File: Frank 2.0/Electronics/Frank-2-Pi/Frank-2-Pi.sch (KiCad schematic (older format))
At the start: 11 parts, among them J2 Left motor, J3 Right motor, Q1 DMN6075S, Q2 DMN6075S, U1 adafruit-2448

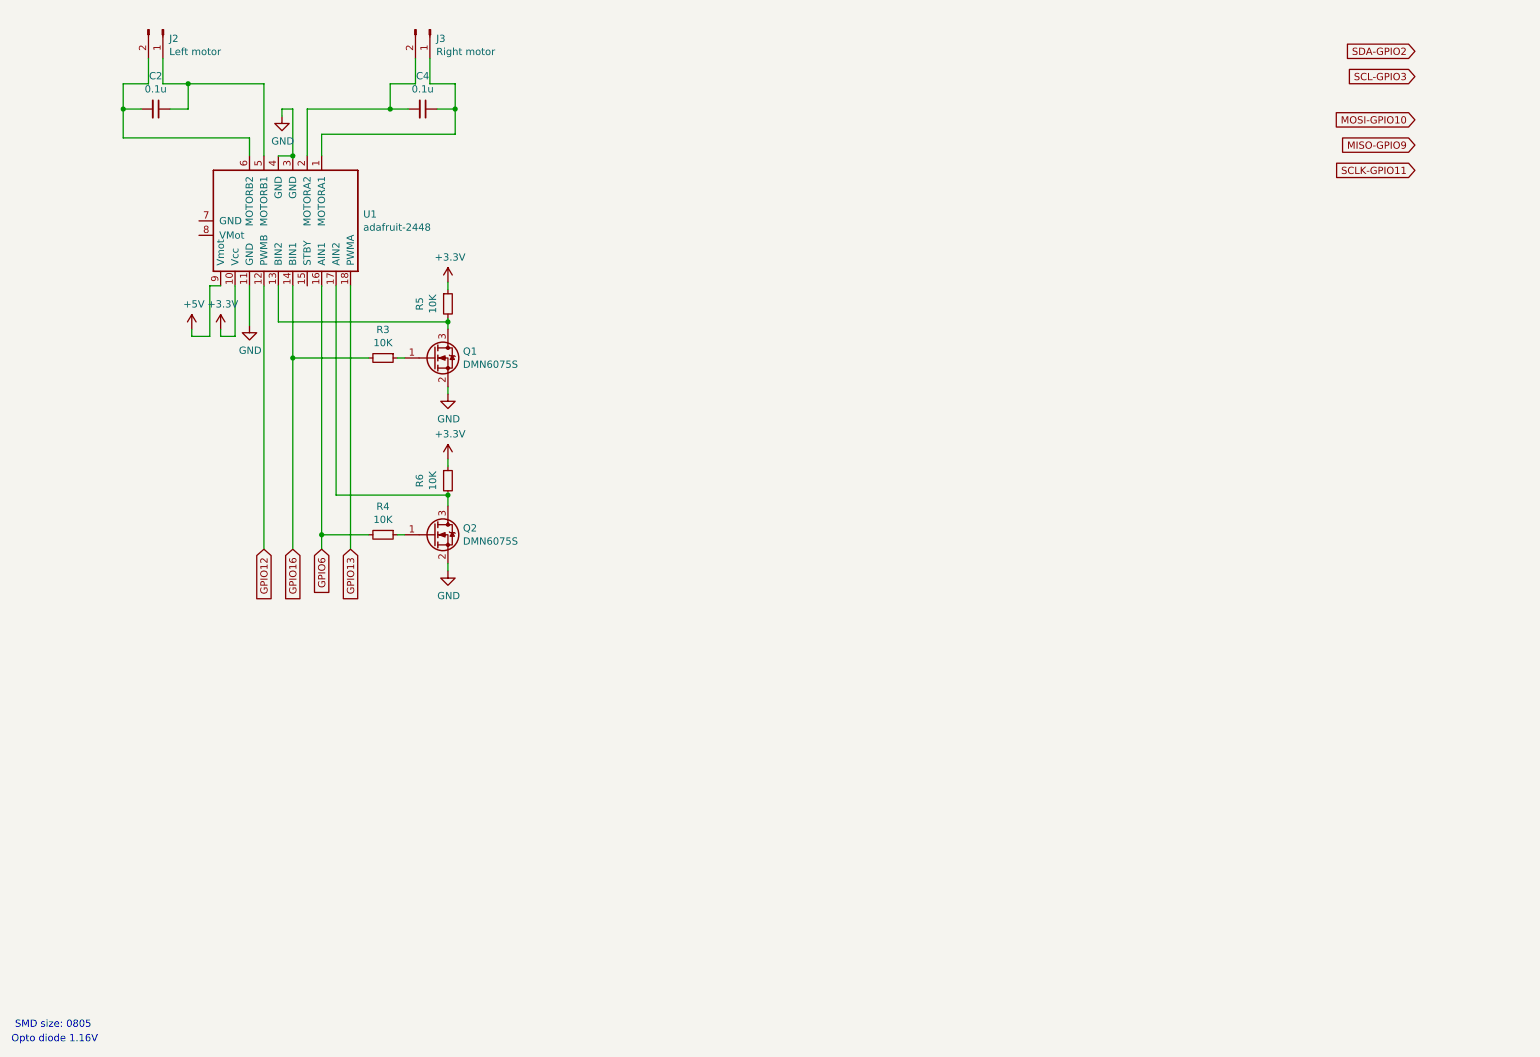
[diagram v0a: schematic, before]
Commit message: Frank 2 electronics WIP.
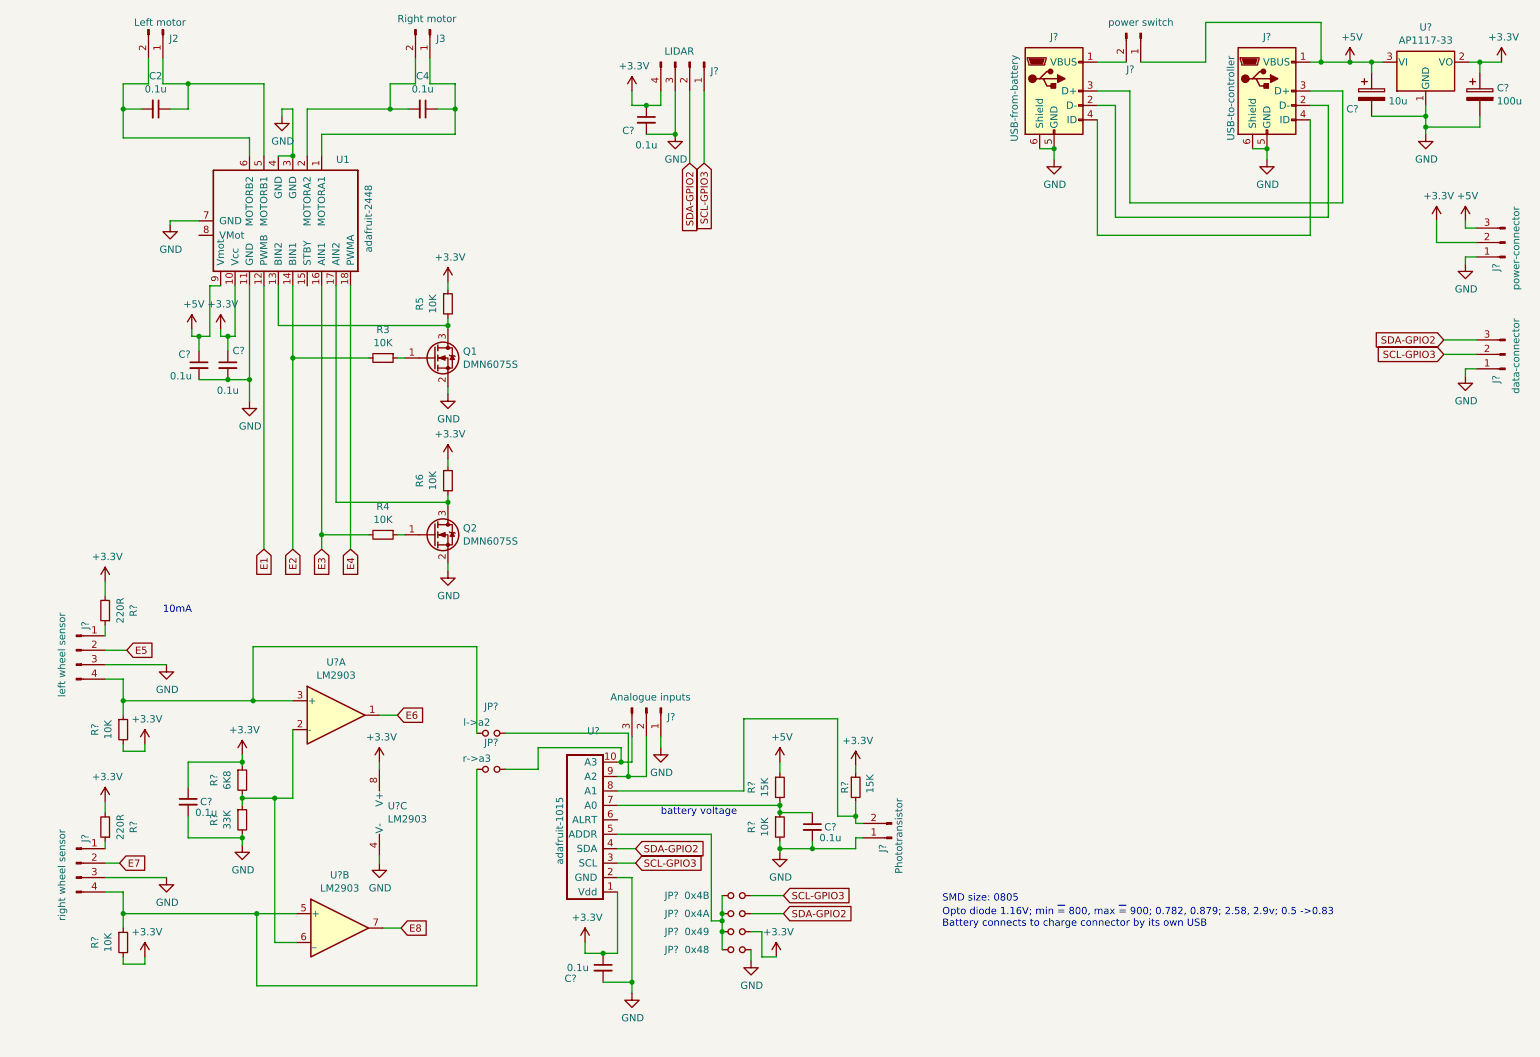
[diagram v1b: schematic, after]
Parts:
- added C? (x6): 0.1u, Capacitor_SMD:C_0805_2012Metric, symbol Device:C_Small
- added C?: 10u, Capacitor_Tantalum_SMD:CP_EIA-3216-18_Kemet-A_Pad1.58x1.35mm_HandSolder, symbol Device:CP
- added C?: 100u, Capacitor_Tantalum_SMD:CP_EIA-3216-18_Kemet-A_Pad1.58x1.35mm_HandSolder, symbol Device:CP
- added J?: LIDAR, Connector_PinHeader_2.54mm:PinHeader_1x04_P2.54mm_Vertical, symbol Connector:Conn_01x04_Male
- added J?: left wheel sensor, Connector_PinHeader_2.54mm:PinHeader_1x04_P2.54mm_Vertical, symbol Connector:Conn_01x04_Male
- added J?: Phototransistor, Connector_PinHeader_2.54mm:PinHeader_1x02_P2.54mm_Vertical, symbol Connector:Conn_01x02_Male
- added J?: Analogue inputs, Connector_PinHeader_2.54mm:PinHeader_1x03_P2.54mm_Vertical, symbol Connector:Conn_01x03_Male
- added J?: right wheel sensor, Connector_PinHeader_2.54mm:PinHeader_1x04_P2.54mm_Vertical, symbol Connector:Conn_01x04_Male
- added J?: USB-to-controller, Connector_USB:USB_Micro-B_Wuerth_629105150521, symbol Connector:USB_OTG
- added J?: USB-from-battery, Connector_USB:USB_Micro-B_Wuerth_629105150521, symbol Connector:USB_OTG
- added J?: power switch, Connector_PinHeader_2.54mm:PinHeader_1x02_P2.54mm_Vertical, symbol Connector:Conn_01x02_Male
- added J?: power-connector, Connector_PinHeader_2.54mm:PinHeader_1x03_P2.54mm_Vertical, symbol Connector:Conn_01x03_Male
- added J?: data-connector, Connector_PinHeader_2.54mm:PinHeader_1x03_P2.54mm_Vertical, symbol Connector:Conn_01x03_Male
- added JP?: 0x48, Jumper:SolderJumper-2_P1.3mm_Open_RoundedPad1.0x1.5mm, symbol Device:Jumper_NO_Small
- added JP?: 0x49, Jumper:SolderJumper-2_P1.3mm_Open_RoundedPad1.0x1.5mm, symbol Device:Jumper_NO_Small
- added JP?: 0x4A, Jumper:SolderJumper-2_P1.3mm_Open_RoundedPad1.0x1.5mm, symbol Device:Jumper_NO_Small
- added JP?: 0x4B, Jumper:SolderJumper-2_P1.3mm_Open_RoundedPad1.0x1.5mm, symbol Device:Jumper_NO_Small
- added JP?: l->a2, Jumper:SolderJumper-2_P1.3mm_Open_RoundedPad1.0x1.5mm, symbol Device:Jumper_NO_Small
- added JP?: r->a3, Jumper:SolderJumper-2_P1.3mm_Open_RoundedPad1.0x1.5mm, symbol Device:Jumper_NO_Small
- added R? (x2): 220R, Resistor_SMD:R_0805_2012Metric, symbol Device:R_Small
- added R? (x3): 10K, Resistor_SMD:R_0805_2012Metric, symbol Device:R_Small
- added R?: 6K8, Resistor_SMD:R_0805_2012Metric, symbol Device:R_Small
- added R?: 33K, Resistor_SMD:R_0805_2012Metric, symbol Device:R_Small
- added R? (x2): 15K, Resistor_SMD:R_0805_2012Metric, symbol Device:R_Small
- added U? (x3): LM2903, Package_SO:Diodes_SO-8EP, symbol Comparator:LM2903
- added U?: adafruit-1015, reprapltd-kicad:adafruit-1015, symbol reprapltd-kicad:adafruit-1015
- added U?: AP1117-33, Package_TO_SOT_SMD:SOT-223-3_TabPin2, symbol Regulator_Linear:AP1117-33
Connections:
- net +3V3: now also C?.1, C?.1, C?.1, C?.1, C?.1, J?.2 (Pin_2), J?.4 (Pin_4), JP?.2, R?.1, R?.1, R?.2, R?.2, R?.2, R?.2, U?.1 (Vdd), U?.2 (VO), U?.8 (V+)
- net +5V: now also C?.1, C?.1, J?.1 (Pin_1), J?.1 (VBUS), J?.3 (Pin_3), R?.1, U?.3 (VI)
- net GND: now also U1.7 (GND), C?.2, C?.2, C?.2, C?.2, C?.2, C?.2, C?.2, C?.2, J?.1 (Pin_1), J?.1 (Pin_1), J?.1 (Pin_1), J?.1 (Pin_1), J?.3 (Pin_3), J?.3 (Pin_3), J?.3 (Pin_3), J?.5 (GND), J?.5 (GND), J?.6 (Shield), J?.6 (Shield), JP?.2, R?.2, R?.2, U?.1 (GND), U?.2 (GND), U?.4 (V-)
- net SCL-GPIO3: now also J?.1 (Pin_1), J?.2 (Pin_2), JP?.2, U?.3 (SCL)
- net SDA-GPIO2: now also J?.2 (Pin_2), J?.3 (Pin_3), JP?.2, U?.4 (SDA)
- net GPIO12 renamed E1
- net GPIO13 renamed E4
- net GPIO16 renamed E2
- net GPIO6 renamed E3
- new net: J?.1 (Pin_1), R?.1 (x2)
- new net: JP?.1, JP?.1, JP?.1, JP?.1, U?.5 (ADDR)
- new net: J?.4 (Pin_4), JP?.1, R?.1, U?.3 (+)
- new net: J?.4 (Pin_4), JP?.1, R?.1, U?.5 (+)
- new net: R?.1, R?.2, U?.2 (-), U?.6 (_)
- new net: J?.3 (Pin_3), JP?.2, U?.10 (A3)
- new net: C?.1, R?.1, R?.2, U?.7 (A0)
- new net: J?.2 (Pin_2), R?.2, U?.8 (A1)
- new net: J?.2 (Pin_2), JP?.2, U?.9 (A2)
- new net: J?.2 (D-), J?.2 (D-)
- new net: J?.3 (D+), J?.3 (D+)
- new net: J?.4 (ID), J?.4 (ID)
- new net: J?.1 (VBUS), J?.2 (Pin_2)
- new net E5: J?.2 (Pin_2)
- new net E6: U?.1
- new net E7: J?.2 (Pin_2)
- new net E8: U?.7
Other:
- note added: "10mA"
- note added: "Opto diode 1.16V; min ~= 800, max ~= 900; 0.782, 0.879; 2.58, 2.9v; 0.5 ->0.83\nBattery connects to charge connector by its own USB"
- note added: "battery voltage"
- note removed: "Opto diode 1.16V"

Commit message: Frank 2.0 electronics WIP.
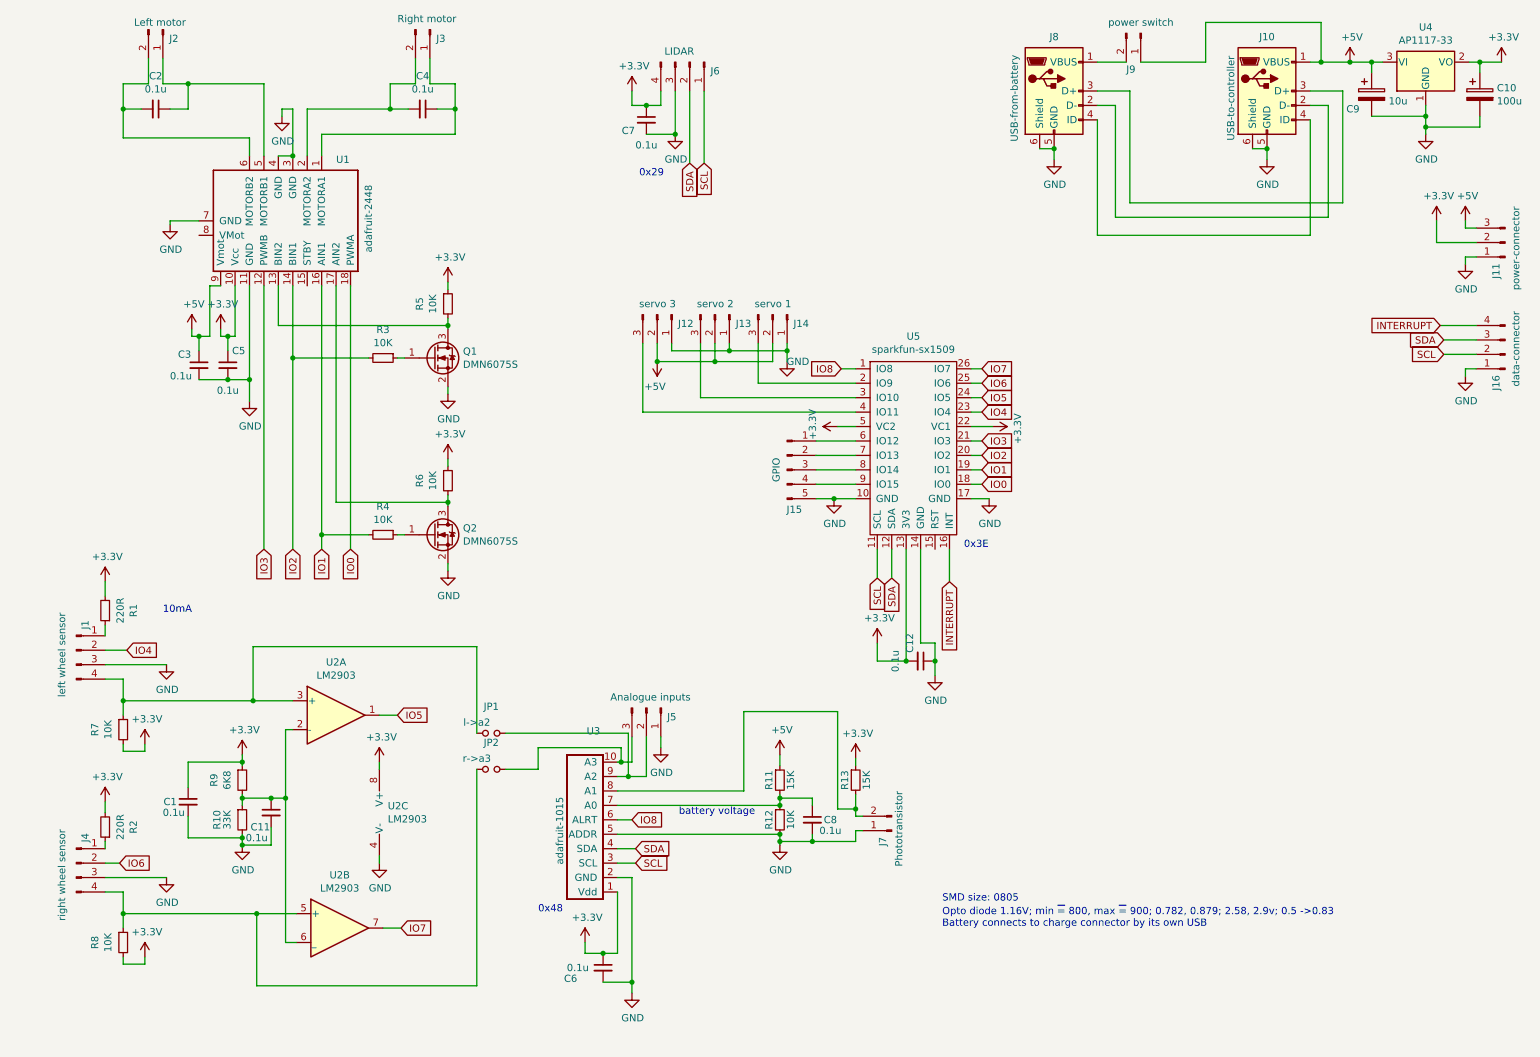
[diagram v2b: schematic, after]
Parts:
- removed J?: data-connector, Connector_PinHeader_2.54mm:PinHeader_1x03_P2.54mm_Vertical, symbol Connector:Conn_01x03_Male
- removed JP?: 0x48, Jumper:SolderJumper-2_P1.3mm_Open_RoundedPad1.0x1.5mm, symbol Device:Jumper_NO_Small
- removed JP?: 0x49, Jumper:SolderJumper-2_P1.3mm_Open_RoundedPad1.0x1.5mm, symbol Device:Jumper_NO_Small
- removed JP?: 0x4A, Jumper:SolderJumper-2_P1.3mm_Open_RoundedPad1.0x1.5mm, symbol Device:Jumper_NO_Small
- removed JP?: 0x4B, Jumper:SolderJumper-2_P1.3mm_Open_RoundedPad1.0x1.5mm, symbol Device:Jumper_NO_Small
- added C11, C12: 0.1u, Capacitor_SMD:C_0805_2012Metric, symbol Device:C_Small
- added J12: servo 3, Connector_PinHeader_2.54mm:PinHeader_1x03_P2.54mm_Vertical, symbol Connector:Conn_01x03_Male
- added J13: servo 2, Connector_PinHeader_2.54mm:PinHeader_1x03_P2.54mm_Vertical, symbol Connector:Conn_01x03_Male
- added J14: servo 1, Connector_PinHeader_2.54mm:PinHeader_1x03_P2.54mm_Vertical, symbol Connector:Conn_01x03_Male
- added J15: GPIO, Connector_PinHeader_2.54mm:PinHeader_1x05_P2.54mm_Vertical, symbol Connector:Conn_01x05_Male
- added J16: data-connector, Connector_PinHeader_2.54mm:PinHeader_1x04_P2.54mm_Vertical, symbol Connector:Conn_01x04_Male
- added U5: sparkfun-sx1509, reprapltd-kicad:sparkfun-sx1509, symbol reprapltd-kicad:sparkfun-sx1509
- gave numbers to parts that had none: 31
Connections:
- net +3V3: now also C12.2, U5.13 (3V3), U5.22 (VC1), U5.5 (VC2)
- net +5V: now also J12.2 (Pin_2), J13.2 (Pin_2), J14.2 (Pin_2)
- net GND: now also U3.5 (ADDR), C11.2, C12.1, J12.1 (Pin_1), J13.1 (Pin_1), J14.1 (Pin_1), J15.5 (Pin_5), J16.1 (Pin_1), U5.10 (GND), U5.14 (GND), U5.17 (GND)
- net at R10.1, R9.2, U2.2 (-)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: now also C11.1
- net IO8: now reaches U3.6 (ALRT)
- net IO8: now also U5.1 (IO8)
- net E1 renamed IO3
- net IO3: now also U5.21 (IO3)
- net E2 renamed IO2
- net IO2: now also U5.20 (IO2)
- net E3 renamed IO1
- net IO1: now also U5.19 (IO1)
- net E4 renamed IO0
- net IO0: now also U5.18 (IO0)
- net E5 renamed IO4
- net IO4: now also U5.23 (IO4)
- net E6 renamed IO5
- net IO5: now also U5.24 (IO5)
- net E7 renamed IO6
- net IO6: now also U5.25 (IO6)
- net E8 renamed IO7
- net IO7: now also U5.26 (IO7)
- net SCL-GPIO3 renamed SCL
- net SCL: now also J16.2 (Pin_2), U5.11 (SCL)
- net SDA-GPIO2 renamed SDA
- net SDA: now also J16.3 (Pin_3), U5.12 (SDA)
- new net: J14.3 (Pin_3), U5.2 (IO9)
- new net: J13.3 (Pin_3), U5.3 (IO10)
- new net: J12.3 (Pin_3), U5.4 (IO11)
- new net: J15.1 (Pin_1), U5.6 (IO12)
- new net: J15.2 (Pin_2), U5.7 (IO13)
- new net: J15.3 (Pin_3), U5.8 (IO14)
- new net: J15.4 (Pin_4), U5.9 (IO15)
- new net INTERRUPT: J16.4 (Pin_4), U5.16 (INT)
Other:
- note added: "0x29"
- note added: "0x3E"
- note added: "0x48"
- moved on the sheet: C8, J7, R11, R12, R13
